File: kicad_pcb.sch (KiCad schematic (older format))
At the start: 162 parts, among them J1 USB_B_Mini, SW1 SW_Push, U1 ATmega32U4-AU, Y1 16Mhz

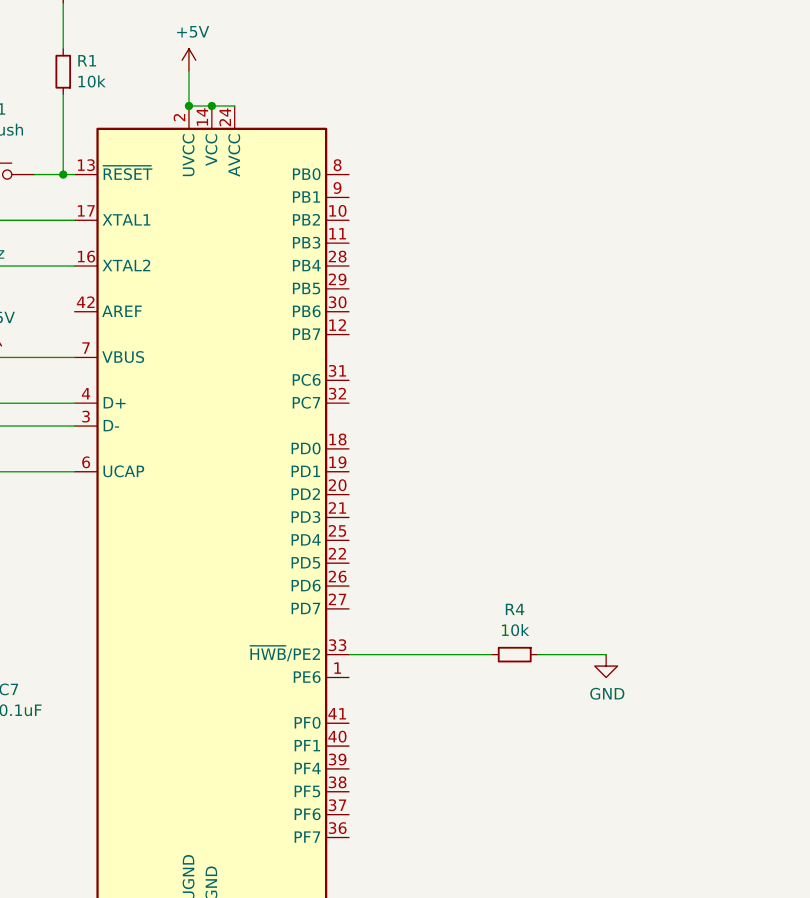
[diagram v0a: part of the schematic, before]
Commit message: further tracing applied
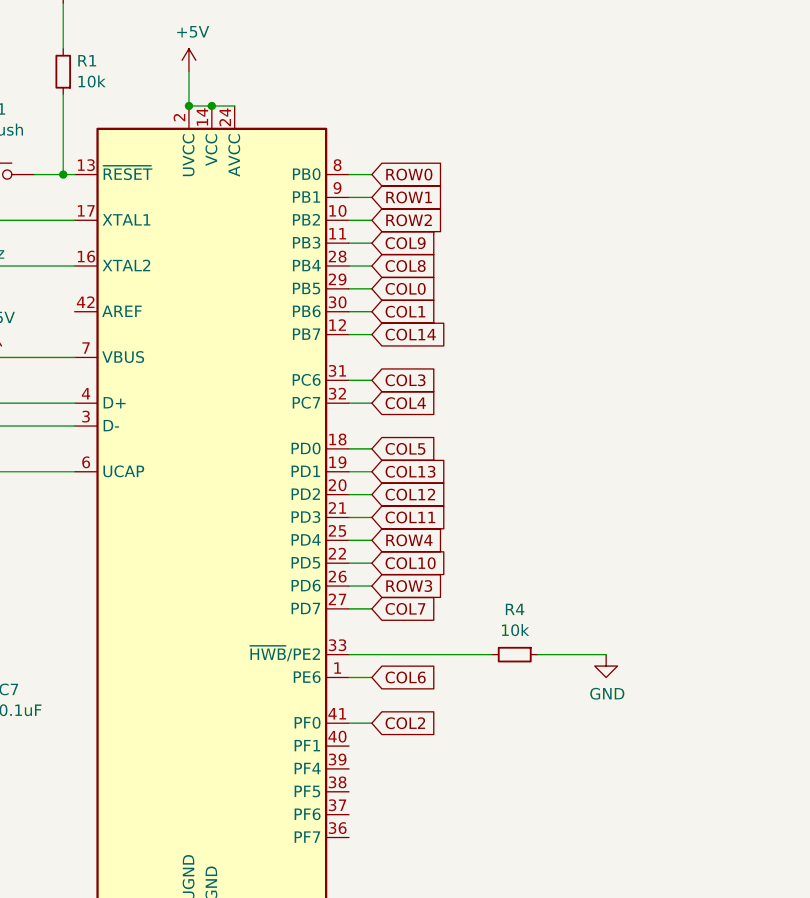
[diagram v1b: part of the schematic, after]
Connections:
- net COL0: now also U1.29 (PB5)
- net COL1: now also U1.30 (PB6)
- net COL10: now also U1.22 (PD5)
- net COL11: now also U1.21 (PD3)
- net COL12: now also U1.20 (PD2)
- net COL13: now also U1.19 (PD1)
- net COL14: now also U1.12 (PB7)
- net COL2: now also U1.41 (PF0)
- net COL3: now also U1.31 (PC6)
- net COL4: now also U1.32 (PC7)
- net COL5: now also U1.18 (PD0)
- net COL6: now also U1.1 (PE6)
- net COL7: now also U1.27 (PD7)
- net COL8: now also U1.28 (PB4)
- net COL9: now also U1.11 (PB3)
- net ROW0: now also U1.8 (PB0)
- net ROW1: now also U1.9 (PB1)
- net ROW2: now also U1.10 (PB2)
- net ROW3: now also U1.26 (PD6)
- net ROW4: now also U1.25 (PD4)
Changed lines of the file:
@@
 $EndDescr
-$Comp
-L MCU_Microchip_ATmega:ATmega32U4-AU U1
-U 1 1 5CCAF324
-P 8775 11800
-F 0 "U1" H 8775 9911 50  0000 C CNN
-F 1 "ATmega32U4-AU" H 8775 9820 50  0000 C CNN
-F 2 "Package_QFP:TQFP-44_10x10mm_P0.8mm" H 8775 11800 50  0001 C CIN
-F 3 "http://ww1.microchip.com/downloads/en/DeviceDoc/Atmel-7766-8-bit-AVR-ATmega16U4-32U4_Datasheet.pdf" H 8775 11800 50  0001 C CNN
-	1    8775 11800
-	1    0    0    -1
-$EndComp
 $Comp
 L Device:R_Small R4
@@
 Wire Wire Line
 	8675 10000 8675 9850
-Wire Wire Line
-	8875 10000 8775 10000
-Connection ~ 8675 10000
-Connection ~ 8775 10000
-Wire Wire Line
-	8775 10000 8675 10000
 $Comp
 L power:GND #PWR0103
@@
 $EndComp
 Wire Wire Line
-	8775 13600 8675 13600
-Connection ~ 8675 13600
-Wire Wire Line
-	8675 13600 8275 13600
-Wire Wire Line
 	10500 12400 10200 12400
-Wire Wire Line
-	10000 12400 9375 12400
 $Comp
 L Device:R_Small R2
@@
 	5000 5050 5000 6050
 Connection ~ 5000 5050
+Text GLabel 9475 12100 2    50   Input ~ 0
+ROW3
+Text GLabel 9475 10500 2    50   Input ~ 0
+ROW2
+Text GLabel 9475 10400 2    50   Input ~ 0
+ROW1
+Text GLabel 9475 10300 2    50   Input ~ 0
+ROW0
+Text GLabel 9475 11700 2    50   Input ~ 0
+COL12
+Text GLabel 9475 11600 2    50   Input ~ 0
+COL13
+Text GLabel 9475 12000 2    50   Input ~ 0
+COL10
+Text GLabel 9475 12200 2    50   Input ~ 0
+COL7
+Text GLabel 9475 11300 2    50   Input ~ 0
+COL4
+Text GLabel 9475 11500 2    50   Input ~ 0
+COL5
+Text GLabel 9475 11200 2    50   Input ~ 0
+COL3
+Text GLabel 9475 10800 2    50   Input ~ 0
+COL0
+Text GLabel 9475 12700 2    50   Input ~ 0
+COL2
+Text GLabel 9475 10900 2    50   Input ~ 0
+COL1
+Connection ~ 8675 13600
+Wire Wire Line
+	8675 13600 8275 13600
+Wire Wire Line
+	8775 13600 8675 13600
+Connection ~ 8775 10000
+Connection ~ 8675 10000
+Wire Wire Line
+	8775 10000 8675 10000
+Wire Wire Line
+	8875 10000 8775 10000
+Wire Wire Line
+	10000 12400 9375 12400
+$Comp
+L MCU_Microchip_ATmega:ATmega32U4-AU U1
+U 1 1 5CCAF324
+P 8775 11800
+F 0 "U1" H 8775 9911 50  0000 C CNN
+F 1 "ATmega32U4-AU" H 8775 9820 50  0000 C CNN
+F 2 "Package_QFP:TQFP-44_10x10mm_P0.8mm" H 8775 11800 50  0001 C CIN
+F 3 "http://ww1.microchip.com/downloads/en/DeviceDoc/Atmel-7766-8-bit-AVR-ATmega16U4-32U4_Datasheet.pdf" H 8775 11800 50  0001 C CNN
+	1    8775 11800
+	1    0    0    -1
+$EndComp
+Text GLabel 9475 11000 2    50   Input ~ 0
+COL14
+Wire Wire Line
+	9375 10400 9475 10400
+Wire Wire Line
+	9475 10300 9375 10300
+Wire Wire Line
+	9375 10500 9475 10500
+Wire Wire Line
+	9475 10600 9375 10600
+Wire Wire Line
+	9375 10700 9475 10700
+Wire Wire Line
+	9475 10800 9375 10800
+Wire Wire Line
+	9375 10900 9475 10900
+Wire Wire Line
+	9475 11000 9375 11000
+Wire Wire Line
+	9375 11200 9475 11200
+Wire Wire Line
+	9475 11300 9375 11300
+Wire Wire Line
+	9375 11500 9475 11500
+Wire Wire Line
+	9375 11700 9475 11700
+Wire Wire Line
+	9375 11900 9475 11900
+Wire Wire Line
+	9375 12000 9475 12000
+Wire Wire Line
+	9375 12200 9475 12200
+Wire Wire Line
+	9375 12500 9475 12500
+Wire Wire Line
+	9475 12700 9375 12700
+Wire Wire Line
+	9475 11800 9375 11800
+Wire Wire Line
+	9475 12100 9375 12100
+Wire Wire Line
+	9475 11600 9375 11600
+Text GLabel 9475 12500 2    50   Input ~ 0
+COL6
+Text GLabel 9475 11900 2    50   Input ~ 0
+ROW4
+Text GLabel 9475 10700 2    50   Input ~ 0
+COL8
+Text GLabel 9475 11800 2    50   Input ~ 0
+COL11
+Text GLabel 9475 10600 2    50   Input ~ 0
+COL9
 $EndSCHEMATC

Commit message: first draft of the v2 PCB completed
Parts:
- MX59: value MX-1U -> SLASH
- MX60: value MX-1U -> R SHIFT
- MX61: value MX-1U -> FN
- MX62: value MX-1U -> CTRL
- MX63: value MX-1U -> WIN
- MX64: value MX-1U -> ALT
- MX65: value MX-1U -> LEFT SPACE; footprint MX_Alps_Hybrid:MXOnly-2.25U-NoLED -> MX_Alps_Hybrid:MXOnly-2.25U-ReversedStabilizers-NoLED
- MX68: value MX-1U -> CENTER
- MX70: value MX-1U -> RIGHT SPACE; footprint MX_Alps_Hybrid:MXOnly-2U-NoLED -> MX_Alps_Hybrid:MXOnly-2U-ReversedStabilizers-NoLED
- MX71: value MX-1U -> LEFT
- MX72: value MX-1U -> DOWN
- MX73: value MX-1U -> UP
- MX74: value MX-1U -> RIGHT
- MX75: value MX-1U -> Fn
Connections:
- net COL0: now also U1.1 (PE6); no longer U1.29 (PB5)
- net COL1: now also U1.41 (PF0); no longer U1.30 (PB6)
- net COL10: now also U1.25 (PD4); no longer U1.22 (PD5)
- net COL11: now also U1.22 (PD5); no longer U1.21 (PD3)
- net COL12: now also U1.21 (PD3); no longer U1.20 (PD2)
- net COL13: now also U1.20 (PD2); no longer U1.19 (PD1)
- net COL14: now also U1.19 (PD1); no longer U1.12 (PB7)
- net COL2: now also U1.40 (PF1); no longer U1.41 (PF0)
- net COL3: now also U1.39 (PF4); no longer U1.31 (PC6)
- net COL4: now also U1.37 (PF6); no longer U1.32 (PC7)
- net COL5: now also U1.36 (PF7); no longer U1.18 (PD0)
- net COL6: now also U1.38 (PF5); no longer U1.1 (PE6)
- net COL7: now also U1.31 (PC6); no longer U1.27 (PD7)
- net COL9: now also U1.26 (PD6); no longer U1.11 (PB3)
- net ROW1: now also U1.18 (PD0); no longer U1.9 (PB1)
- net ROW2: now also U1.29 (PB5); no longer U1.10 (PB2)
- net ROW3: now also U1.12 (PB7); no longer U1.26 (PD6)
- net ROW4: now also U1.30 (PB6); no longer U1.25 (PD4)
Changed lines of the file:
@@
 P 21075 6075
 F 0 "MX75" H 21161 6292 60  0000 C CNN
-F 1 "MX-1U" H 21161 6218 20  0000 C CNN
+F 1 "Fn" H 21161 6218 20  0000 C CNN
 F 2 "MX_Alps_Hybrid:MXOnly-1U-NoLED" H 21050 6050 60  0001 C CNN
 F 3 "" H 21050 6050 60  0001 C CNN
@@
 P 19825 6075
 F 0 "MX74" H 19911 6292 60  0000 C CNN
-F 1 "MX-1U" H 19911 6218 20  0000 C CNN
+F 1 "RIGHT" H 19911 6218 20  0000 C CNN
 F 2 "MX_Alps_Hybrid:MXOnly-1U-NoLED" H 19800 6050 60  0001 C CNN
 F 3 "" H 19800 6050 60  0001 C CNN
@@
 P 18575 6075
 F 0 "MX73" H 18661 6292 60  0000 C CNN
-F 1 "MX-1U" H 18661 6218 20  0000 C CNN
+F 1 "UP" H 18661 6218 20  0000 C CNN
 F 2 "MX_Alps_Hybrid:MXOnly-1U-NoLED" H 18550 6050 60  0001 C CNN
 F 3 "" H 18550 6050 60  0001 C CNN
@@
 P 17325 6075
 F 0 "MX72" H 17411 6292 60  0000 C CNN
-F 1 "MX-1U" H 17411 6218 20  0000 C CNN
+F 1 "DOWN" H 17411 6218 20  0000 C CNN
 F 2 "MX_Alps_Hybrid:MXOnly-1U-NoLED" H 17300 6050 60  0001 C CNN
 F 3 "" H 17300 6050 60  0001 C CNN
@@
 P 16075 6075
 F 0 "MX71" H 16161 6292 60  0000 C CNN
-F 1 "MX-1U" H 16161 6218 20  0000 C CNN
+F 1 "LEFT" H 16161 6218 20  0000 C CNN
 F 2 "MX_Alps_Hybrid:MXOnly-1U-NoLED" H 16050 6050 60  0001 C CNN
 F 3 "" H 16050 6050 60  0001 C CNN
@@
 P 14825 6075
 F 0 "MX70" H 14911 6292 60  0000 C CNN
-F 1 "MX-1U" H 14911 6218 20  0000 C CNN
-F 2 "MX_Alps_Hybrid:MXOnly-2U-NoLED" H 14800 6050 60  0001 C CNN
+F 1 "RIGHT SPACE" H 14911 6218 20  0000 C CNN
+F 2 "MX_Alps_Hybrid:MXOnly-2U-ReversedStabilizers-NoLED" H 14800 6050 60  0001 C CNN
 F 3 "" H 14800 6050 60  0001 C CNN
 	1    14825 6075
@@
 P 12325 6075
 F 0 "MX68" H 12411 6292 60  0000 C CNN
-F 1 "MX-1U" H 12411 6218 20  0000 C CNN
+F 1 "CENTER" H 12411 6218 20  0000 C CNN
 F 2 "MX_Alps_Hybrid:MXOnly-1U-NoLED" H 12300 6050 60  0001 C CNN
 F 3 "" H 12300 6050 60  0001 C CNN
@@
 P 8575 6075
 F 0 "MX65" H 8661 6292 60  0000 C CNN
-F 1 "MX-1U" H 8661 6218 20  0000 C CNN
-F 2 "MX_Alps_Hybrid:MXOnly-2.25U-NoLED" H 8550 6050 60  0001 C CNN
+F 1 "LEFT SPACE" H 8661 6218 20  0000 C CNN
+F 2 "MX_Alps_Hybrid:MXOnly-2.25U-ReversedStabilizers-NoLED" H 8550 6050 60  0001 C CNN
 F 3 "" H 8550 6050 60  0001 C CNN
 	1    8575 6075
@@
 P 7325 6075
 F 0 "MX64" H 7411 6292 60  0000 C CNN
-F 1 "MX-1U" H 7411 6218 20  0000 C CNN
+F 1 "ALT" H 7411 6218 20  0000 C CNN
 F 2 "MX_Alps_Hybrid:MXOnly-1.25U-NoLED" H 7300 6050 60  0001 C CNN
 F 3 "" H 7300 6050 60  0001 C CNN
@@
 P 4825 6075
 F 0 "MX62" H 4911 6292 60  0000 C CNN
-F 1 "MX-1U" H 4911 6218 20  0000 C CNN
+F 1 "CTRL" H 4911 6218 20  0000 C CNN
 F 2 "MX_Alps_Hybrid:MXOnly-1.25U-NoLED" H 4800 6050 60  0001 C CNN
 F 3 "" H 4800 6050 60  0001 C CNN
@@
 P 3575 6075
 F 0 "MX61" H 3661 6292 60  0000 C CNN
-F 1 "MX-1U" H 3661 6218 20  0000 C CNN
+F 1 "FN" H 3661 6218 20  0000 C CNN
 F 2 "MX_Alps_Hybrid:MXOnly-1U-NoLED" H 3550 6050 60  0001 C CNN
 F 3 "" H 3550 6050 60  0001 C CNN
@@
 P 6075 6075
 F 0 "MX63" H 6161 6292 60  0000 C CNN
-F 1 "MX-1U" H 6161 6218 20  0000 C CNN
+F 1 "WIN" H 6161 6218 20  0000 C CNN
 F 2 "MX_Alps_Hybrid:MXOnly-1.25U-NoLED" H 6050 6050 60  0001 C CNN
 F 3 "" H 6050 6050 60  0001 C CNN
@@
 P 21075 5075
 F 0 "MX60" H 21161 5292 60  0000 C CNN
-F 1 "MX-1U" H 21161 5218 20  0000 C CNN
+F 1 "R SHIFT" H 21161 5218 20  0000 C CNN
 F 2 "MX_Alps_Hybrid:MXOnly-1U-NoLED" H 21050 5050 60  0001 C CNN
 F 3 "" H 21050 5050 60  0001 C CNN
@@
 P 19825 5075
 F 0 "MX59" H 19911 5292 60  0000 C CNN
-F 1 "MX-1U" H 19911 5218 20  0000 C CNN
+F 1 "SLASH" H 19911 5218 20  0000 C CNN
 F 2 "MX_Alps_Hybrid:MXOnly-1U-NoLED" H 19800 5050 60  0001 C CNN
 F 3 "" H 19800 5050 60  0001 C CNN
@@
 	5000 5050 5000 6050
 Connection ~ 5000 5050
-Text GLabel 9475 12100 2    50   Input ~ 0
-ROW3
-Text GLabel 9475 10500 2    50   Input ~ 0
+Text GLabel 9475 10800 2    50   Input ~ 0
 ROW2
-Text GLabel 9475 10400 2    50   Input ~ 0
-ROW1
 Text GLabel 9475 10300 2    50   Input ~ 0
 ROW0
+Text GLabel 9475 11800 2    50   Input ~ 0
+COL12
 Text GLabel 9475 11700 2    50   Input ~ 0
-COL12
-Text GLabel 9475 11600 2    50   Input ~ 0
 COL13
-Text GLabel 9475 12000 2    50   Input ~ 0
+Text GLabel 9475 11900 2    50   Input ~ 0
 COL10
-Text GLabel 9475 12200 2    50   Input ~ 0
-COL7
-Text GLabel 9475 11300 2    50   Input ~ 0
+Text GLabel 9475 13100 2    50   Input ~ 0
 COL4
-Text GLabel 9475 11500 2    50   Input ~ 0
+Text GLabel 9475 13200 2    50   Input ~ 0
 COL5
-Text GLabel 9475 11200 2    50   Input ~ 0
+Text GLabel 9475 12900 2    50   Input ~ 0
 COL3
-Text GLabel 9475 10800 2    50   Input ~ 0
+Text GLabel 9475 12500 2    50   Input ~ 0
 COL0
+Text GLabel 9475 12800 2    50   Input ~ 0
+COL2
 Text GLabel 9475 12700 2    50   Input ~ 0
-COL2
-Text GLabel 9475 10900 2    50   Input ~ 0
 COL1
 Connection ~ 8675 13600
@@
 	1    0    0    -1
 $EndComp
-Text GLabel 9475 11000 2    50   Input ~ 0
+Text GLabel 9475 11600 2    50   Input ~ 0
 COL14
 Wire Wire Line
@@
 Wire Wire Line
 	9475 11600 9375 11600
-Text GLabel 9475 12500 2    50   Input ~ 0
+Text GLabel 9475 13000 2    50   Input ~ 0
 COL6
-Text GLabel 9475 11900 2    50   Input ~ 0
-ROW4
 Text GLabel 9475 10700 2    50   Input ~ 0
 COL8
-Text GLabel 9475 11800 2    50   Input ~ 0
+Wire Wire Line
+	9475 12800 9375 12800
+Wire Wire Line
+	9375 12900 9475 12900
+Wire Wire Line
+	9475 13000 9375 13000
+Wire Wire Line
+	9375 13100 9475 13100
+Wire Wire Line
+	9475 13200 9375 13200
+Text GLabel 9475 10900 2    50   Input ~ 0
+ROW4
+Text GLabel 9475 11000 2    50   Input ~ 0
+ROW3
+Text GLabel 9475 12100 2    50   Input ~ 0
+COL9
+Text GLabel 9475 12000 2    50   Input ~ 0
 COL11
-Text GLabel 9475 10600 2    50   Input ~ 0
-COL9
+Text GLabel 9475 11200 2    50   Input ~ 0
+COL7
+Text GLabel 9475 11500 2    50   Input ~ 0
+ROW1
 $EndSCHEMATC

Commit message: ready to export
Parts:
- C1, C2, C3, C4, C5, C6: footprint Capacitor_SMD:C_0201_0603Metric -> Capacitor_SMD:C_0805_2012Metric
- R2, R3: footprint Resistor_SMD:R_0603_1608Metric -> Resistor_SMD:R_0805_2012Metric
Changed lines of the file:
@@
 F 0 "R2" V 6879 11300 50  0000 C CNN
 F 1 "22" V 6970 11300 50  0000 C CNN
-F 2 "Resistor_SMD:R_0603_1608Metric" H 7075 11300 50  0001 C CNN
+F 2 "Resistor_SMD:R_0805_2012Metric" H 7075 11300 50  0001 C CNN
 F 3 "~" H 7075 11300 50  0001 C CNN
 	1    7075 11300
@@
 F 0 "R3" V 6604 11400 50  0000 C CNN
 F 1 "22" V 6695 11400 50  0000 C CNN
-F 2 "Resistor_SMD:R_0603_1608Metric" H 6800 11400 50  0001 C CNN
+F 2 "Resistor_SMD:R_0805_2012Metric" H 6800 11400 50  0001 C CNN
 F 3 "~" H 6800 11400 50  0001 C CNN
 	1    6800 11400
@@
 F 0 "C3" H 7667 11746 50  0000 L CNN
 F 1 "1uF" H 7667 11655 50  0000 L CNN
-F 2 "Capacitor_SMD:C_0201_0603Metric" H 7575 11700 50  0001 C CNN
+F 2 "Capacitor_SMD:C_0805_2012Metric" H 7575 11700 50  0001 C CNN
 F 3 "~" H 7575 11700 50  0001 C CNN
 	1    7575 11700
@@
 F 0 "C5" H 6842 12646 50  0000 L CNN
 F 1 "0.1uF" H 6842 12555 50  0000 L CNN
-F 2 "Capacitor_SMD:C_0201_0603Metric" H 6750 12600 50  0001 C CNN
+F 2 "Capacitor_SMD:C_0805_2012Metric" H 6750 12600 50  0001 C CNN
 F 3 "~" H 6750 12600 50  0001 C CNN
 	1    6750 12600
@@
 F 0 "C6" H 7342 12646 50  0000 L CNN
 F 1 "0.1uF" H 7342 12555 50  0000 L CNN
-F 2 "Capacitor_SMD:C_0201_0603Metric" H 7250 12600 50  0001 C CNN
+F 2 "Capacitor_SMD:C_0805_2012Metric" H 7250 12600 50  0001 C CNN
 F 3 "~" H 7250 12600 50  0001 C CNN
 	1    7250 12600
@@
 F 0 "C4" H 6342 12646 50  0000 L CNN
 F 1 "0.1uF" H 6342 12555 50  0000 L CNN
-F 2 "Capacitor_SMD:C_0201_0603Metric" H 6250 12600 50  0001 C CNN
+F 2 "Capacitor_SMD:C_0805_2012Metric" H 6250 12600 50  0001 C CNN
 F 3 "~" H 6250 12600 50  0001 C CNN
 	1    6250 12600
@@
 F 0 "C1" V 6871 10425 50  0000 C CNN
 F 1 "22pF" V 6962 10425 50  0000 C CNN
-F 2 "Capacitor_SMD:C_0201_0603Metric" H 7100 10425 50  0001 C CNN
+F 2 "Capacitor_SMD:C_0805_2012Metric" H 7100 10425 50  0001 C CNN
 F 3 "~" H 7100 10425 50  0001 C CNN
 	1    7100 10425
@@
 F 0 "C2" V 6871 10775 50  0000 C CNN
 F 1 "22pF" V 6962 10775 50  0000 C CNN
-F 2 "Capacitor_SMD:C_0201_0603Metric" H 7100 10775 50  0001 C CNN
+F 2 "Capacitor_SMD:C_0805_2012Metric" H 7100 10775 50  0001 C CNN
 F 3 "~" H 7100 10775 50  0001 C CNN
 	1    7100 10775
